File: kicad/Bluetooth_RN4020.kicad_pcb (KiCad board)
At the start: 2 copper layers, 10 parts, among them U1 RN4020

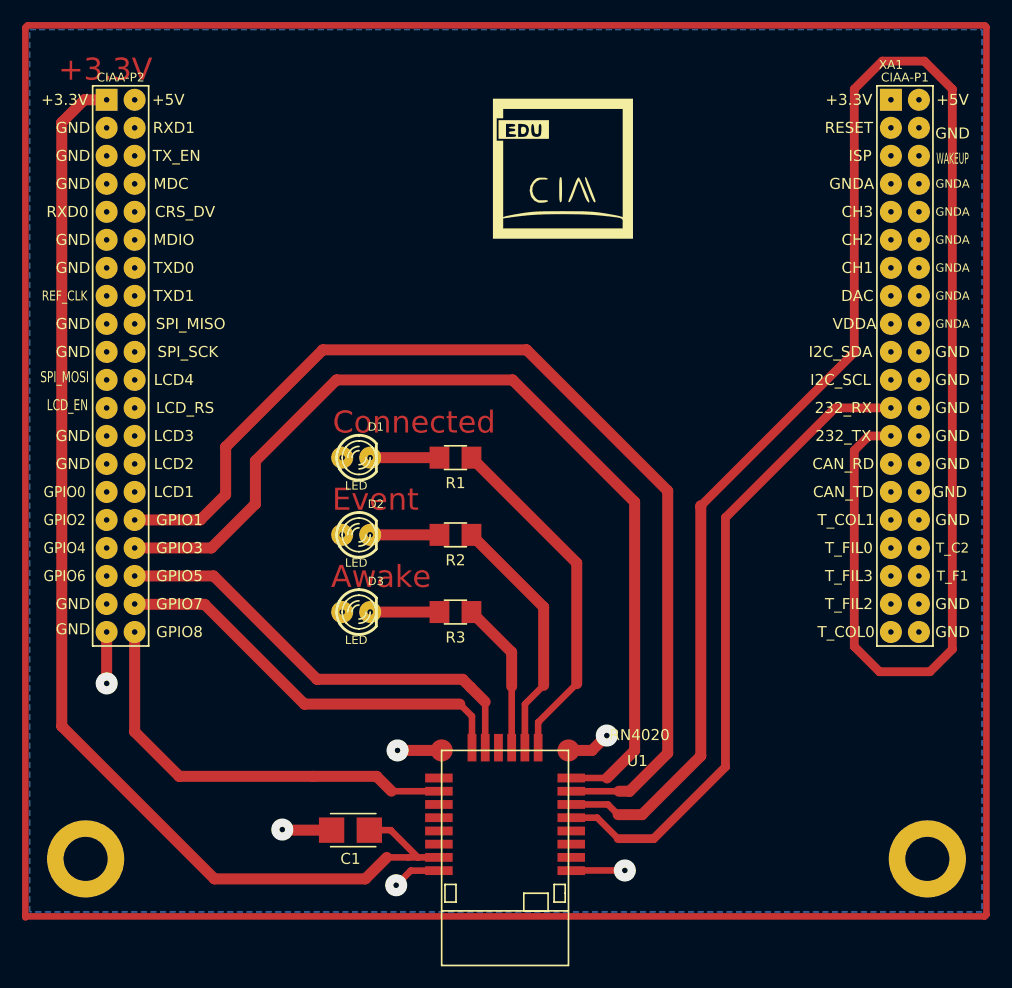
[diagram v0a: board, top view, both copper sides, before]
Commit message: Kicad Fix
Fix the Kicad
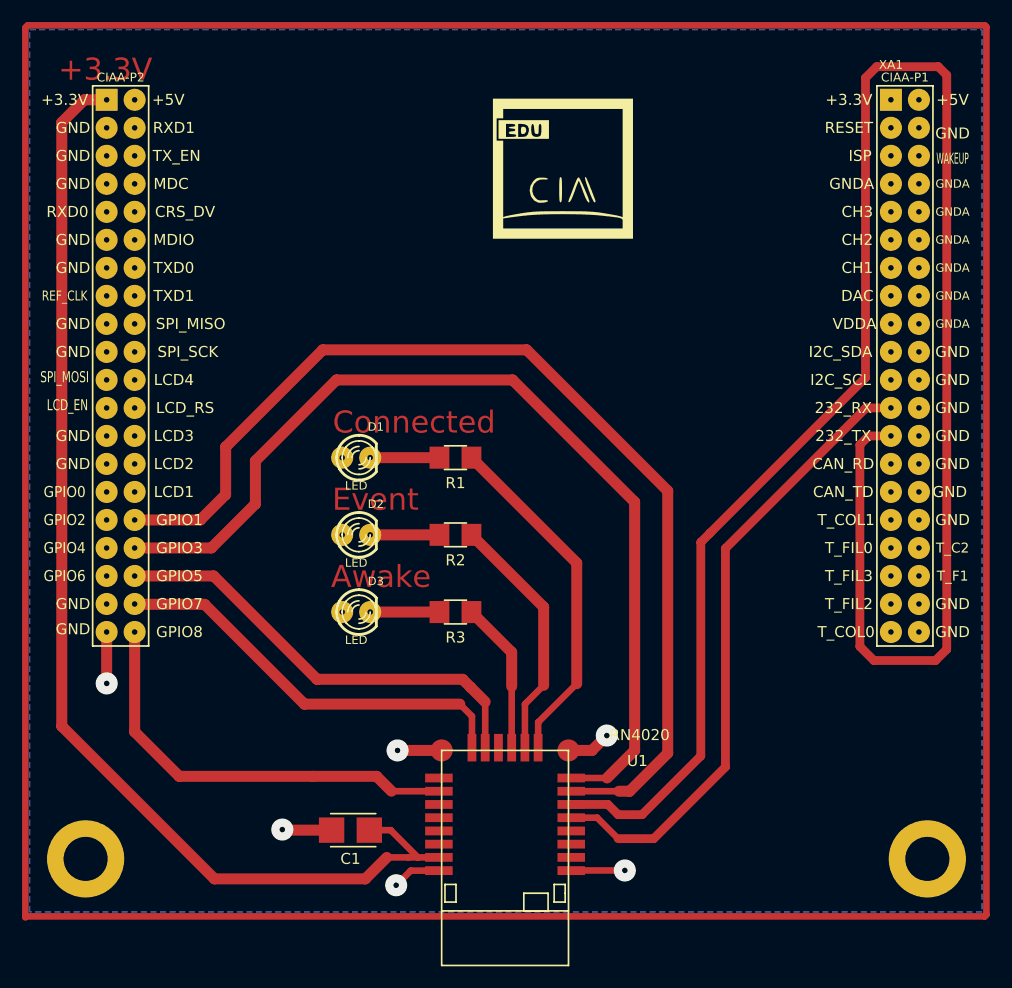
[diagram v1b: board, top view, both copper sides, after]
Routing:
- net TX: track 174.8 -> 172.4 mm
- net RX: track 59.2 -> 57.6 mm
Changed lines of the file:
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@@
     (links 23)
     (no_connects 0)
-    (area 0 0 0 0)
+    (area 106.349999 57.849999 194.300002 143.675001)
     (thickness 1.6)
     (drawings 4)
-    (tracks 121)
+    (tracks 120)
     (zones 0)
     (modules 10)
@@
   (segment (start 161.55 127.7) (end 165 124.25) (width 1) (layer F.Cu) (net 22))
   (segment (start 160.57 127.7) (end 161.55 127.7) (width 1) (layer F.Cu) (net 22))
-  (segment (start 168 101.876) (end 168 101.824) (width 0.8) (layer F.Cu) (net 23))
-  (segment (start 183.234 95.48) (end 185.24 95.48) (width 0.8) (layer F.Cu) (net 23) (status 800000))
-  (segment (start 181.918 96.796) (end 183.234 95.48) (width 0.8) (layer F.Cu) (net 23))
-  (segment (start 181.918 114.576) (end 181.918 96.796) (width 0.8) (layer F.Cu) (net 23))
-  (segment (start 184.204 116.862) (end 181.918 114.576) (width 0.8) (layer F.Cu) (net 23))
-  (segment (start 188.776 116.862) (end 184.204 116.862) (width 0.8) (layer F.Cu) (net 23))
-  (segment (start 190.808 114.83) (end 188.776 116.862) (width 0.8) (layer F.Cu) (net 23))
-  (segment (start 190.808 64.03) (end 190.808 114.83) (width 0.8) (layer F.Cu) (net 23))
-  (segment (start 188.268 61.49) (end 190.808 64.03) (width 0.8) (layer F.Cu) (net 23))
-  (segment (start 184.458 61.49) (end 188.268 61.49) (width 0.8) (layer F.Cu) (net 23))
-  (segment (start 181.918 64.03) (end 184.458 61.49) (width 0.8) (layer F.Cu) (net 23))
-  (segment (start 181.918 87.906) (end 181.918 64.03) (width 0.8) (layer F.Cu) (net 23))
-  (segment (start 168 101.824) (end 181.918 87.906) (width 0.8) (layer F.Cu) (net 23))
-  (segment (start 168 124.5) (end 168 101.876) (width 1) (layer F.Cu) (net 23))
-  (segment (start 168 101.876) (end 168 101.80066) (width 1) (layer F.Cu) (net 23))
-  (segment (start 160.5 129.8252) (end 162.6748 129.8252) (width 1) (layer F.Cu) (net 23))
-  (segment (start 159.5748 128.9) (end 160.5 129.8252) (width 0.6) (layer F.Cu) (net 23))
-  (segment (start 156.25 128.9) (end 159.5748 128.9) (width 0.6) (layer F.Cu) (net 23))
-  (segment (start 162.6748 129.8252) (end 168 124.5) (width 1) (layer F.Cu) (net 23))
+  (segment (start 168 124.5) (end 168 105.126) (width 0.8) (layer F.Cu) (net 23))
+  (segment (start 162.6748 129.8252) (end 168 124.5) (width 0.8) (layer F.Cu) (net 23))
+  (segment (start 156.25 128.9) (end 159.5748 128.9) (width 0.8) (layer F.Cu) (net 23))
+  (segment (start 159.5748 128.9) (end 160.5 129.8252) (width 0.8) (layer F.Cu) (net 23))
+  (segment (start 160.5 129.8252) (end 162.6748 129.8252) (width 0.8) (layer F.Cu) (net 23))
+  (segment (start 168.837 104.289) (end 182.934 90.192) (width 0.8) (layer F.Cu) (net 23))
+  (segment (start 168 105.126) (end 168.837 104.289) (width 0.8) (layer F.Cu) (net 23))
+  (segment (start 182.934 90.192) (end 182.934 63.014) (width 0.8) (layer F.Cu) (net 23))
+  (segment (start 182.934 63.014) (end 183.95 61.998) (width 0.8) (layer F.Cu) (net 23))
+  (segment (start 183.95 61.998) (end 189.538 61.998) (width 0.8) (layer F.Cu) (net 23))
+  (segment (start 189.538 61.998) (end 190.3 62.76) (width 0.8) (layer F.Cu) (net 23))
+  (segment (start 190.3 62.76) (end 190.3 114.83) (width 0.8) (layer F.Cu) (net 23))
+  (segment (start 190.3 114.83) (end 189.284 115.846) (width 0.8) (layer F.Cu) (net 23))
+  (segment (start 189.284 115.846) (end 183.696 115.846) (width 0.8) (layer F.Cu) (net 23))
+  (segment (start 183.696 115.846) (end 182.426 114.576) (width 0.8) (layer F.Cu) (net 23))
+  (segment (start 182.426 114.576) (end 182.426 96.288) (width 0.8) (layer F.Cu) (net 23))
+  (segment (start 182.426 96.288) (end 183.234 95.48) (width 0.8) (layer F.Cu) (net 23))
+  (segment (start 183.234 95.48) (end 185.24 95.48) (width 0.8) (layer F.Cu) (net 23))
   (segment (start 160.5 132) (end 163.732 132) (width 0.8) (layer F.Cu) (net 24))
   (segment (start 158.6 130.1) (end 160.5 132) (width 0.6) (layer F.Cu) (net 24))
   (segment (start 156.25 130.1) (end 158.6 130.1) (width 0.6) (layer F.Cu) (net 24))
-  (segment (start 180.186 92.94) (end 185.24 92.94) (width 0.8) (layer F.Cu) (net 24) (status 800000))
-  (segment (start 170.234 102.892) (end 180.186 92.94) (width 0.8) (layer F.Cu) (net 24))
-  (segment (start 170.234 125.498) (end 170.234 102.892) (width 0.8) (layer F.Cu) (net 24))
+  (segment (start 182.98 92.94) (end 185.24 92.94) (width 0.8) (layer F.Cu) (net 24) (status 800000))
+  (segment (start 170.234 105.686) (end 182.98 92.94) (width 0.8) (layer F.Cu) (net 24))
+  (segment (start 170.234 125.498) (end 170.234 105.686) (width 0.8) (layer F.Cu) (net 24))
   (segment (start 163.732 132) (end 170.234 125.498) (width 0.8) (layer F.Cu) (net 24))
   (segment (start 156.25 126.5) (end 159.5 126.5) (width 0.6) (layer F.Cu) (net 25))
